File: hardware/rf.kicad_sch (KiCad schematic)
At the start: 83 parts, among them J4 SMA-KWE901, J5 SMA-KWE901, U11 MT7603E, X1 HSO321S-50MHZ-3.3V

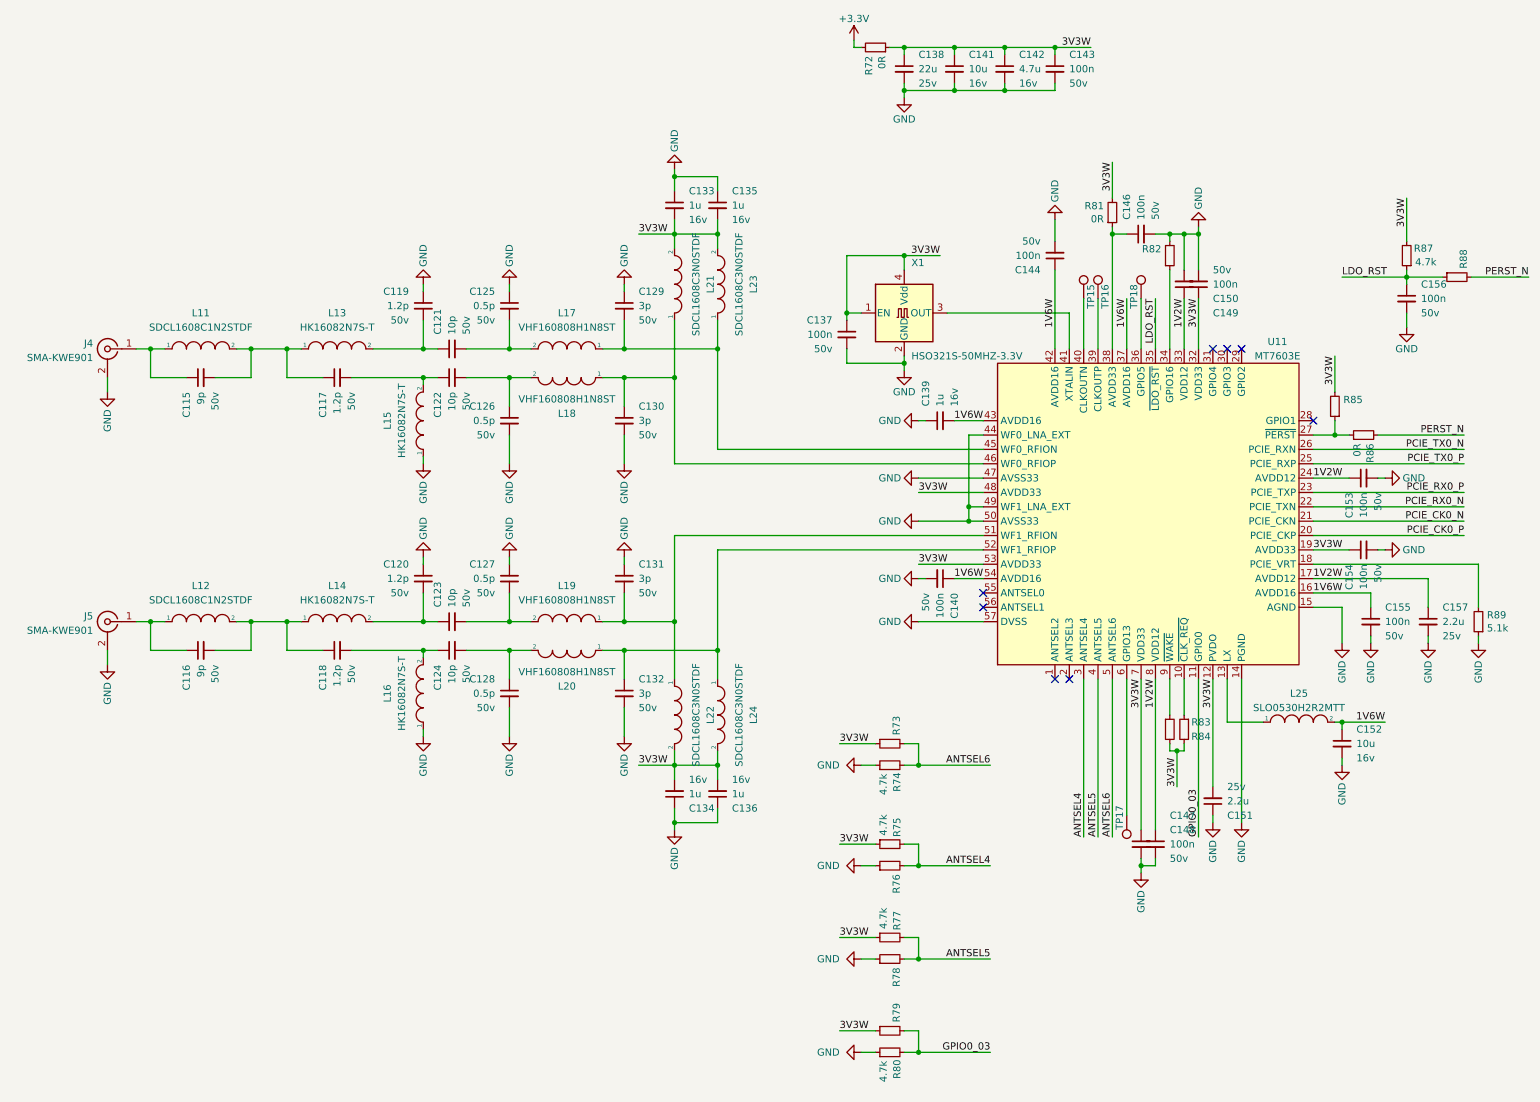
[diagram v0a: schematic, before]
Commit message: update cap and dru
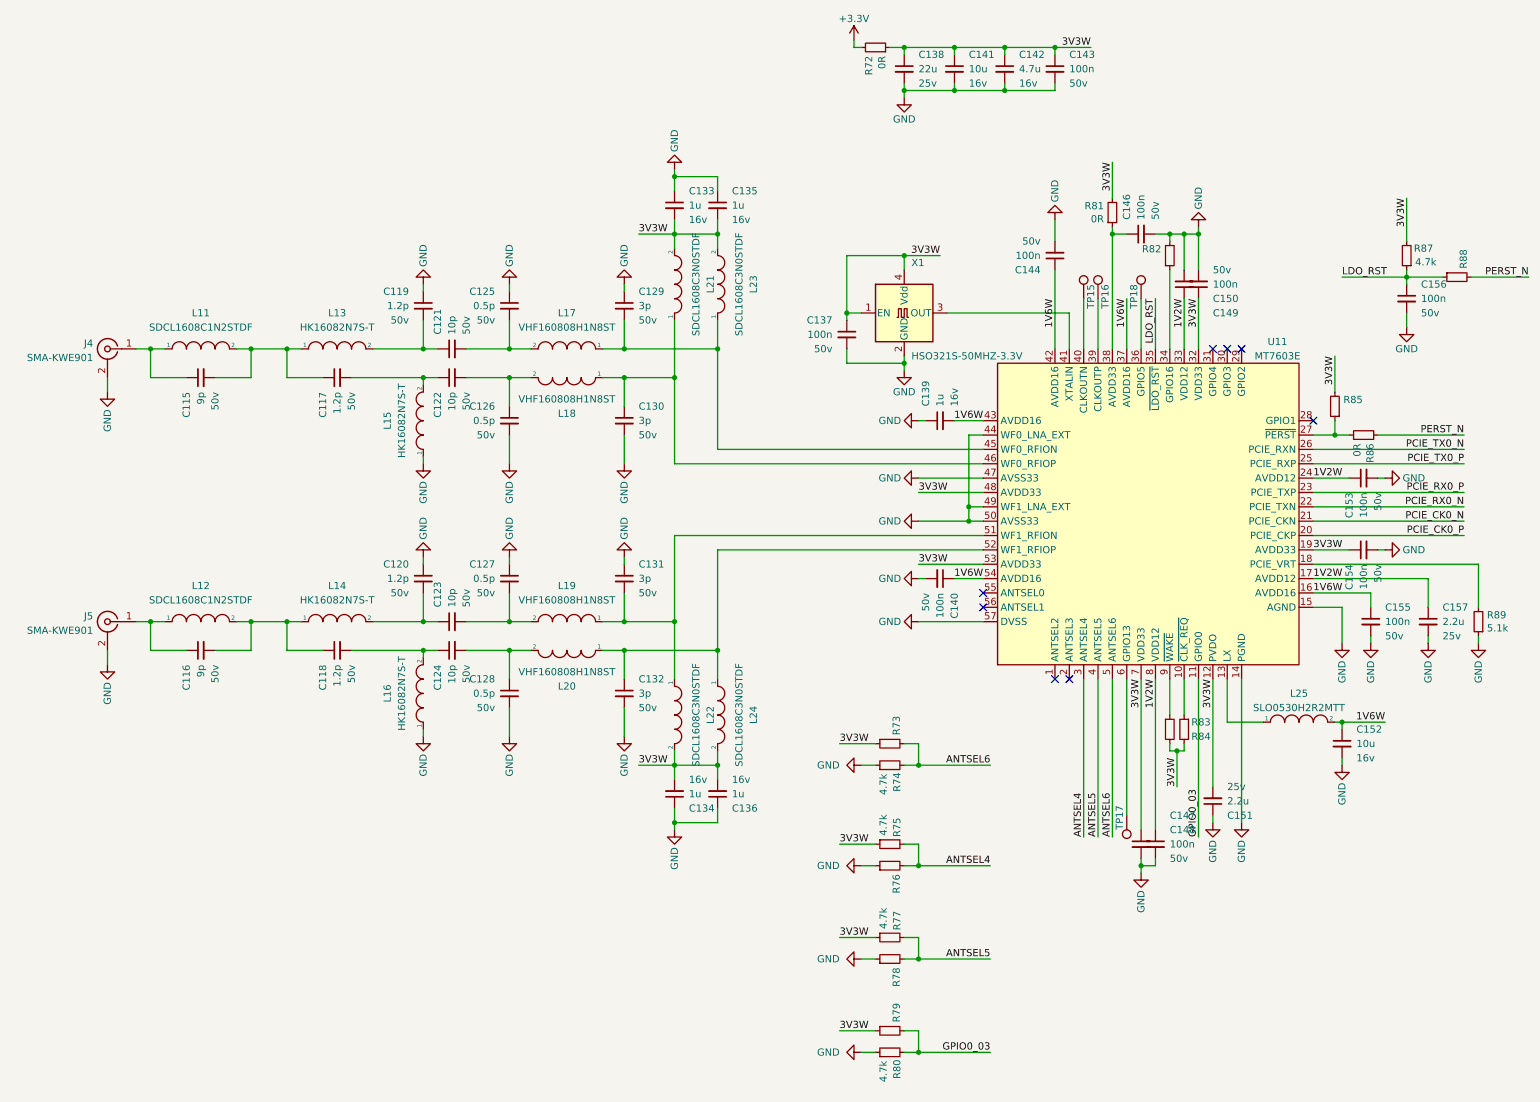
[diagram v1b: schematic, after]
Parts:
- C115, C116: footprint Capacitor_SMD:C_0603_1608Metric -> Capacitor_SMD:C_0402_1005Metric; lcsc C282076 -> C88899
- C117, C118, C119, C120: footprint Capacitor_SMD:C_0603_1608Metric -> Capacitor_SMD:C_0402_1005Metric; lcsc C437533 -> C72135
- C121, C122, C123, C124: footprint Capacitor_SMD:C_0603_1608Metric -> Capacitor_SMD:C_0402_1005Metric; lcsc C1634 -> C32949
- C125, C126, C127, C128: footprint Capacitor_SMD:C_0603_1608Metric -> Capacitor_SMD:C_0402_1005Metric; lcsc C1633 -> C76912
- C129, C130, C131, C132: footprint Capacitor_SMD:C_0603_1608Metric -> Capacitor_SMD:C_0402_1005Metric; lcsc C46219 -> C88891
- C137, C140, C143, C144, C146, C147, C148, C149, C150, C153, C154, C155, C156: footprint Capacitor_SMD:C_0603_1608Metric -> Capacitor_SMD:C_0402_1005Metric; lcsc C14663 -> C307331
- R72, R81, R86: footprint Resistor_SMD:R_0603_1608Metric -> Resistor_SMD:R_0402_1005Metric; lcsc C21189 -> C17168
- R73, R76, R78, R79, R82, R83, R84, R85, R88: footprint Resistor_SMD:R_0603_1608Metric -> Resistor_SMD:R_0402_1005Metric
- R74, R75, R77, R80, R87: footprint Resistor_SMD:R_0603_1608Metric -> Resistor_SMD:R_0402_1005Metric; lcsc C23162 -> C25900
- R89: footprint Resistor_SMD:R_0603_1608Metric -> Resistor_SMD:R_0402_1005Metric; lcsc C23186 -> C25905
